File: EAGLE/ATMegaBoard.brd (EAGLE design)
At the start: 77.5 x 55.5 mm, 29 parts, among them IC1 L298, IC2 ATMEGA168-20P, IC3 REG1117, X1 49S/18PF

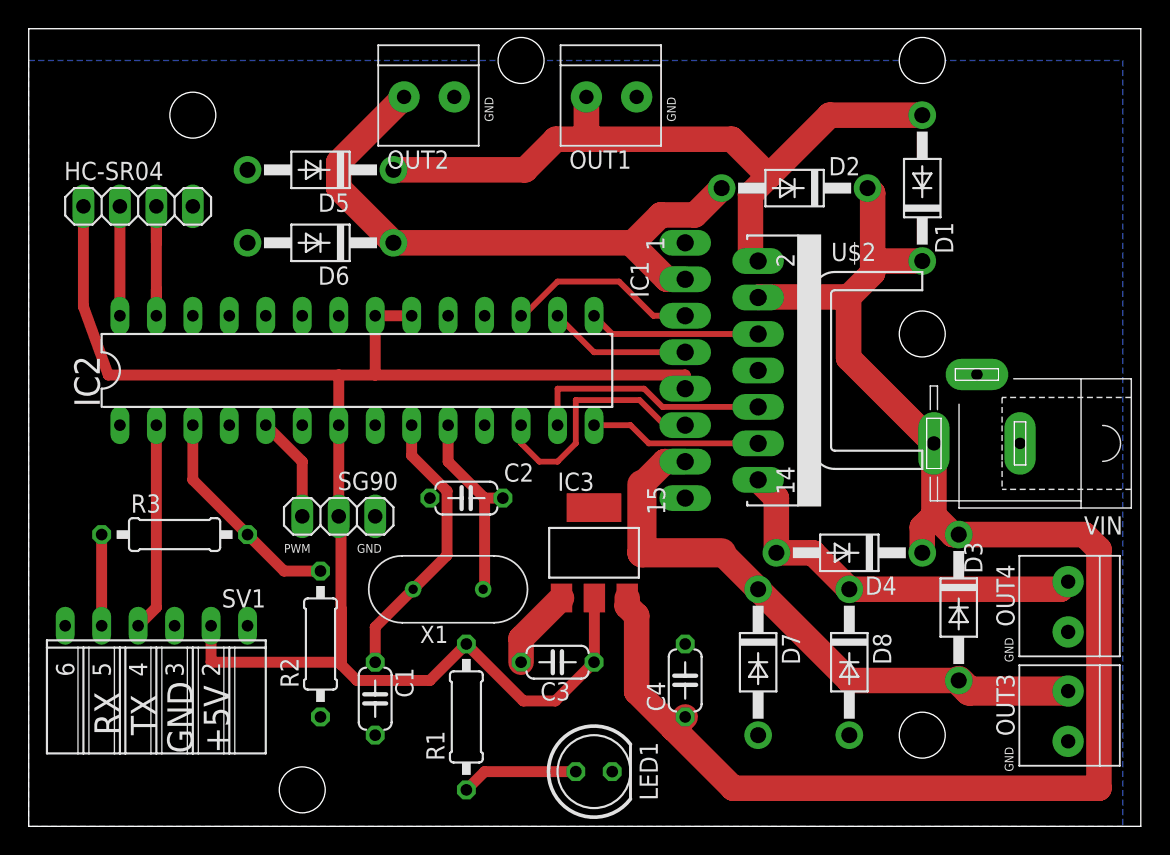
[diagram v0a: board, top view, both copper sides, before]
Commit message: compressed board
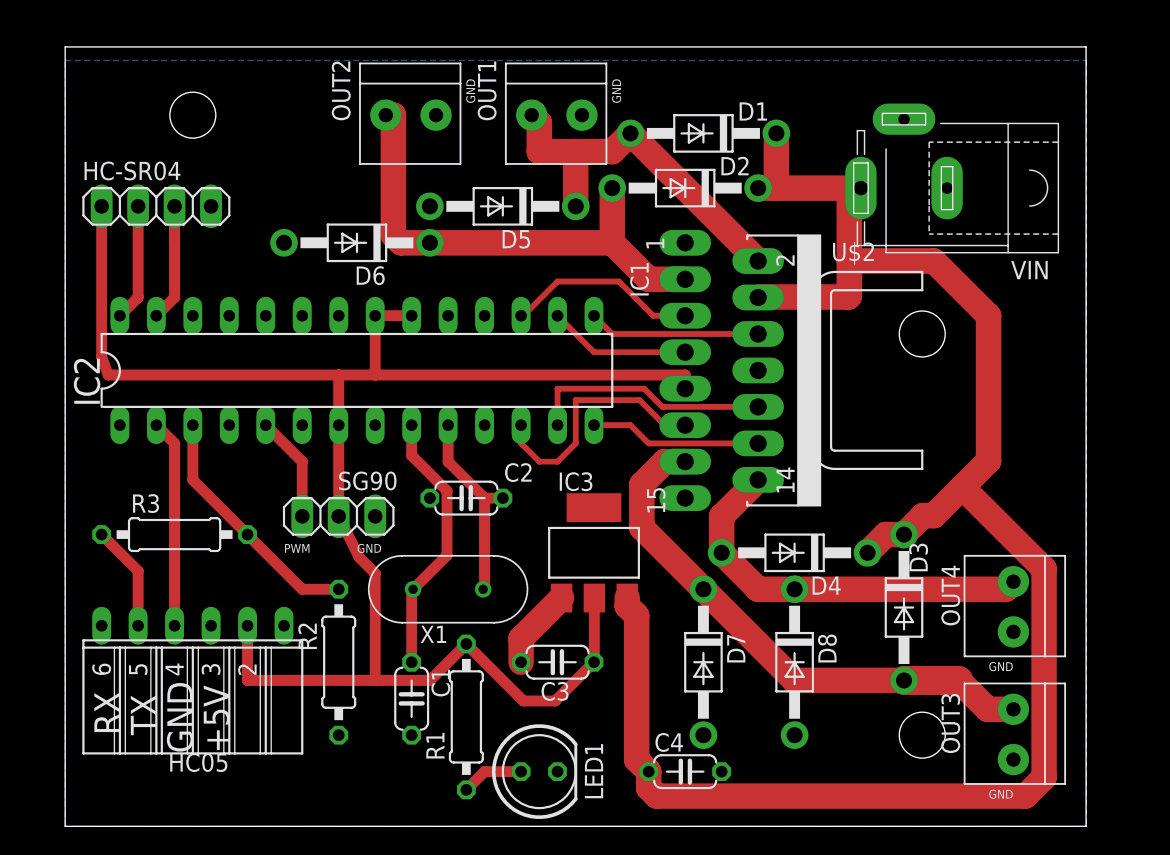
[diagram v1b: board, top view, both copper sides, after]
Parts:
- removed SV1: (no value), con-lsta:FE06W
- added HC05: (no value), con-lsta:FE06W
- moved VIN 18.5 mm to (64.8, 45.7)
- moved D1 15.7 mm to (50.8, 49.5), turned to 180 degrees
- moved D5 13.0 mm to (36.8, 44.5)
- moved D2 7.62 mm to (49.5, 45.7)
- moved C4 6.35 mm to (49.5, 5.08), turned to 0 degrees
- moved OUT1 4.02 mm to (40.6, 50.8)
- moved OUT3 4.02 mm to (72.4, 7.62)
- moved D3 3.81 mm to (64.8, 16.5)
- moved D4 3.81 mm to (57.1, 20.3)
- moved D7 3.81 mm to (50.8, 12.7)
- moved D8 3.81 mm to (57.1, 12.7)
- moved LED1 3.81 mm to (39.4, 5.08)
- moved OUT4 3.81 mm to (72.4, 16.5)
- moved D6 2.54 mm to (26.7, 41.9)
- moved C1 2.54 mm to (30.5, 10.2)
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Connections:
- net +5V: now also HC05.2; no longer SV1.2
- net GND: now also HC05.3; no longer SV1.3
- net PIN5HC05: now also HC05.5; no longer SV1.5
- net TX: now also HC05.4; no longer SV1.4
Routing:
- net OUT1: track 50.4 -> 26.0 mm
- net VIN: track 110.8 -> 122.1 mm
- net OUT2: track 42.9 -> 34.3 mm
- net OUT3: track 42.1 -> 37.8 mm
- net +5V: track 121.8 -> 117.9 mm
- net N$3: track 8.15 -> 4.34 mm
- net RX: track 15.3 -> 17.1 mm
- net ECHO: track 12.0 -> 10.7 mm
- net XTAL1: track 19.6 -> 18.6 mm
- net PIN5HC05: track 6.35 -> 7.40 mm
- net TRIG: track 7.62 -> 8.15 mm
- net OUT4: track 27.2 -> 27.7 mm
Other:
- board size 77.5 x 55.5 mm -> 71.1 x 54.3 mm
